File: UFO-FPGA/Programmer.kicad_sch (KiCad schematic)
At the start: 38 parts, among them U2 FT2232HL, U3 ASDMB-12MHz, U5 93LC56CT-I/MS

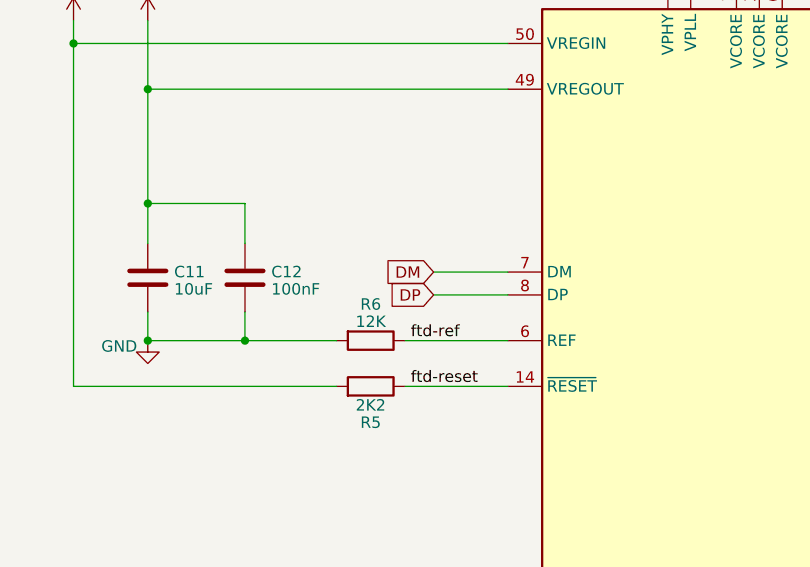
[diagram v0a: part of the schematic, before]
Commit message: pcb prog redesign
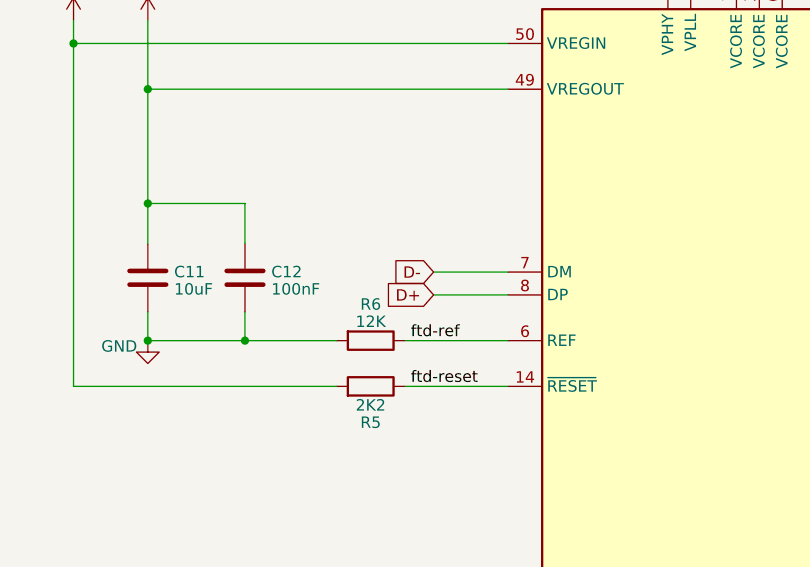
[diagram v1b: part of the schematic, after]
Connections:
- net DM renamed D-
- net DP renamed D+
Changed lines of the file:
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@@
     )
   )
-  (global_label "DP" (shape input) (at 215.265 109.22 180) (fields_autoplaced)
+  (global_label "D+" (shape input) (at 215.265 109.22 180) (fields_autoplaced)
     (effects (font (size 1.27 1.27)) (justify right))
-    (property "Intersheetrefs" "${INTERSHEET_REFS}" (at 209.8192 109.22 0)
+    (property "Intersheetrefs" "${INTERSHEET_REFS}" (at 209.5168 109.22 0)
       (effects (font (size 1.27 1.27)) (justify right) hide)
     )
@@
     )
   )
-  (global_label "DM" (shape input) (at 215.265 106.68 180) (fields_autoplaced)
+  (global_label "D-" (shape input) (at 215.265 106.68 180) (fields_autoplaced)
     (effects (font (size 1.27 1.27)) (justify right))
-    (property "Intersheetrefs" "${INTERSHEET_REFS}" (at 209.6378 106.68 0)
+    (property "Intersheetrefs" "${INTERSHEET_REFS}" (at 209.5168 106.68 0)
       (effects (font (size 1.27 1.27)) (justify right) hide)
     )

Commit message: pcb 0603
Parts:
- C1, C12, C13, C2, C3, C4, C7, C8: footprint Capacitor_SMD:C_0805_2012Metric_Pad1.18x1.45mm_HandSolder -> Capacitor_SMD:C_0603_1608Metric_Pad1.08x0.95mm_HandSolder
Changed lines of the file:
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@@
       (effects (font (size 1.27 1.27)) (justify left))
     )
-    (property "Footprint" "Capacitor_SMD:C_0805_2012Metric_Pad1.18x1.45mm_HandSolder" (at 207.3402 36.83 0)
+    (property "Footprint" "Capacitor_SMD:C_0603_1608Metric_Pad1.08x0.95mm_HandSolder" (at 207.3402 36.83 0)
       (effects (font (size 1.27 1.27)) hide)
     )
@@
       (effects (font (size 1.27 1.27)) (justify right))
     )
-    (property "Footprint" "Capacitor_SMD:C_0805_2012Metric_Pad1.18x1.45mm_HandSolder" (at 249.8598 37.465 0)
+    (property "Footprint" "Capacitor_SMD:C_0603_1608Metric_Pad1.08x0.95mm_HandSolder" (at 249.8598 37.465 0)
       (effects (font (size 1.27 1.27)) hide)
     )
@@
       (effects (font (size 1.27 1.27)) (justify left))
     )
-    (property "Footprint" "Capacitor_SMD:C_0805_2012Metric_Pad1.18x1.45mm_HandSolder" (at 198.4502 36.83 0)
+    (property "Footprint" "Capacitor_SMD:C_0603_1608Metric_Pad1.08x0.95mm_HandSolder" (at 198.4502 36.83 0)
       (effects (font (size 1.27 1.27)) hide)
     )
@@
       (effects (font (size 1.27 1.27)) (justify left))
     )
-    (property "Footprint" "Capacitor_SMD:C_0805_2012Metric_Pad1.18x1.45mm_HandSolder" (at 195.2752 111.125 0)
+    (property "Footprint" "Capacitor_SMD:C_0603_1608Metric_Pad1.08x0.95mm_HandSolder" (at 195.2752 111.125 0)
       (effects (font (size 1.27 1.27)) hide)
     )
@@
       (effects (font (size 1.27 1.27)) (justify left))
     )
-    (property "Footprint" "Capacitor_SMD:C_0805_2012Metric_Pad1.18x1.45mm_HandSolder" (at 86.0552 160.02 0)
+    (property "Footprint" "Capacitor_SMD:C_0603_1608Metric_Pad1.08x0.95mm_HandSolder" (at 86.0552 160.02 0)
       (effects (font (size 1.27 1.27)) hide)
     )
@@
       (effects (font (size 1.27 1.27)) (justify left))
     )
-    (property "Footprint" "Capacitor_SMD:C_0805_2012Metric_Pad1.18x1.45mm_HandSolder" (at 180.0352 175.895 0)
+    (property "Footprint" "Capacitor_SMD:C_0603_1608Metric_Pad1.08x0.95mm_HandSolder" (at 180.0352 175.895 0)
       (effects (font (size 1.27 1.27)) hide)
     )
@@
       (effects (font (size 1.27 1.27)) (justify left))
     )
-    (property "Footprint" "Capacitor_SMD:C_0805_2012Metric_Pad1.18x1.45mm_HandSolder" (at 189.5602 36.83 0)
+    (property "Footprint" "Capacitor_SMD:C_0603_1608Metric_Pad1.08x0.95mm_HandSolder" (at 189.5602 36.83 0)
       (effects (font (size 1.27 1.27)) hide)
     )
@@
       (effects (font (size 1.27 1.27)) (justify left))
     )
-    (property "Footprint" "Capacitor_SMD:C_0805_2012Metric_Pad1.18x1.45mm_HandSolder" (at 232.7402 36.83 0)
-      (effects (font (size 1.27 1.27)) hide)
-    )
+    (property "Footprint" "Capacitor_SMD:C_0603_1608Metric_Pad1.08x0.95mm_HandSolder" (at 232.7402 36.83 0)
+      (effects (font (size 1.27 1.27)) hide)
+    )

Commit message: pcb and footprints
0603
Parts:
- R10, R11, R12, R13, R14, R15, R16, R17, R18, R19, R20, R7, R8, R9: footprint Resistor_SMD:R_0805_2012Metric_Pad1.20x1.40mm_HandSolder -> Resistor_SMD:R_0603_1608Metric_Pad0.98x0.95mm_HandSolder
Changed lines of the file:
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@@
       (effects (font (size 1.27 1.27)))
     )
-    (property "Footprint" "Resistor_SMD:R_0805_2012Metric_Pad1.20x1.40mm_HandSolder" (at 307.34 144.018 90)
+    (property "Footprint" "Resistor_SMD:R_0603_1608Metric_Pad0.98x0.95mm_HandSolder" (at 307.34 144.018 90)
       (effects (font (size 1.27 1.27)) hide)
     )
@@
       (effects (font (size 1.27 1.27)))
     )
-    (property "Footprint" "Resistor_SMD:R_0805_2012Metric_Pad1.20x1.40mm_HandSolder" (at 307.34 100.838 90)
+    (property "Footprint" "Resistor_SMD:R_0603_1608Metric_Pad0.98x0.95mm_HandSolder" (at 307.34 100.838 90)
       (effects (font (size 1.27 1.27)) hide)
     )
@@
       (effects (font (size 1.27 1.27)))
     )
-    (property "Footprint" "Resistor_SMD:R_0805_2012Metric_Pad1.20x1.40mm_HandSolder" (at 307.34 131.318 90)
+    (property "Footprint" "Resistor_SMD:R_0603_1608Metric_Pad0.98x0.95mm_HandSolder" (at 307.34 131.318 90)
       (effects (font (size 1.27 1.27)) hide)
     )
@@
       (effects (font (size 1.27 1.27)))
     )
-    (property "Footprint" "Resistor_SMD:R_0805_2012Metric_Pad1.20x1.40mm_HandSolder" (at 307.34 93.218 90)
+    (property "Footprint" "Resistor_SMD:R_0603_1608Metric_Pad0.98x0.95mm_HandSolder" (at 307.34 93.218 90)
       (effects (font (size 1.27 1.27)) hide)
     )
@@
       (effects (font (size 1.27 1.27)))
     )
-    (property "Footprint" "Resistor_SMD:R_0805_2012Metric_Pad1.20x1.40mm_HandSolder" (at 307.34 128.778 90)
+    (property "Footprint" "Resistor_SMD:R_0603_1608Metric_Pad0.98x0.95mm_HandSolder" (at 307.34 128.778 90)
       (effects (font (size 1.27 1.27)) hide)
     )
@@
       (effects (font (size 1.27 1.27)))
     )
-    (property "Footprint" "Resistor_SMD:R_0805_2012Metric_Pad1.20x1.40mm_HandSolder" (at 307.34 85.598 90)
+    (property "Footprint" "Resistor_SMD:R_0603_1608Metric_Pad0.98x0.95mm_HandSolder" (at 307.34 85.598 90)
       (effects (font (size 1.27 1.27)) hide)
     )
@@
       (effects (font (size 1.27 1.27)))
     )
-    (property "Footprint" "Resistor_SMD:R_0805_2012Metric_Pad1.20x1.40mm_HandSolder" (at 307.34 88.138 90)
+    (property "Footprint" "Resistor_SMD:R_0603_1608Metric_Pad0.98x0.95mm_HandSolder" (at 307.34 88.138 90)
       (effects (font (size 1.27 1.27)) hide)
     )
@@
       (effects (font (size 1.27 1.27)))
     )
-    (property "Footprint" "Resistor_SMD:R_0805_2012Metric_Pad1.20x1.40mm_HandSolder" (at 307.34 83.058 90)
+    (property "Footprint" "Resistor_SMD:R_0603_1608Metric_Pad0.98x0.95mm_HandSolder" (at 307.34 83.058 90)
       (effects (font (size 1.27 1.27)) hide)
     )
@@
       (effects (font (size 1.27 1.27)))
     )
-    (property "Footprint" "Resistor_SMD:R_0805_2012Metric_Pad1.20x1.40mm_HandSolder" (at 307.34 138.938 90)
+    (property "Footprint" "Resistor_SMD:R_0603_1608Metric_Pad0.98x0.95mm_HandSolder" (at 307.34 138.938 90)
       (effects (font (size 1.27 1.27)) hide)
     )
@@
       (effects (font (size 1.27 1.27)))
     )
-    (property "Footprint" "Resistor_SMD:R_0805_2012Metric_Pad1.20x1.40mm_HandSolder" (at 184.785 193.548 90)
+    (property "Footprint" "Resistor_SMD:R_0603_1608Metric_Pad0.98x0.95mm_HandSolder" (at 184.785 193.548 90)
       (effects (font (size 1.27 1.27)) hide)
     )
@@
       (effects (font (size 1.27 1.27)))
     )
-    (property "Footprint" "Resistor_SMD:R_0805_2012Metric_Pad1.20x1.40mm_HandSolder" (at 307.34 141.478 90)
+    (property "Footprint" "Resistor_SMD:R_0603_1608Metric_Pad0.98x0.95mm_HandSolder" (at 307.34 141.478 90)
       (effects (font (size 1.27 1.27)) hide)
     )
@@
       (effects (font (size 1.27 1.27)))
     )
-    (property "Footprint" "Resistor_SMD:R_0805_2012Metric_Pad1.20x1.40mm_HandSolder" (at 307.34 98.298 90)
+    (property "Footprint" "Resistor_SMD:R_0603_1608Metric_Pad0.98x0.95mm_HandSolder" (at 307.34 98.298 90)
       (effects (font (size 1.27 1.27)) hide)
     )
@@
       (effects (font (size 1.27 1.27)))
     )
-    (property "Footprint" "Resistor_SMD:R_0805_2012Metric_Pad1.20x1.40mm_HandSolder" (at 307.34 133.858 90)
+    (property "Footprint" "Resistor_SMD:R_0603_1608Metric_Pad0.98x0.95mm_HandSolder" (at 307.34 133.858 90)
       (effects (font (size 1.27 1.27)) hide)
     )
@@
       (effects (font (size 1.27 1.27)))
     )
-    (property "Footprint" "Resistor_SMD:R_0805_2012Metric_Pad1.20x1.40mm_HandSolder" (at 307.34 136.398 90)
-      (effects (font (size 1.27 1.27)) hide)
-    )
+    (property "Footprint" "Resistor_SMD:R_0603_1608Metric_Pad0.98x0.95mm_HandSolder" (at 307.34 136.398 90)
+      (effects (font (size 1.27 1.27)) hide)
+    )

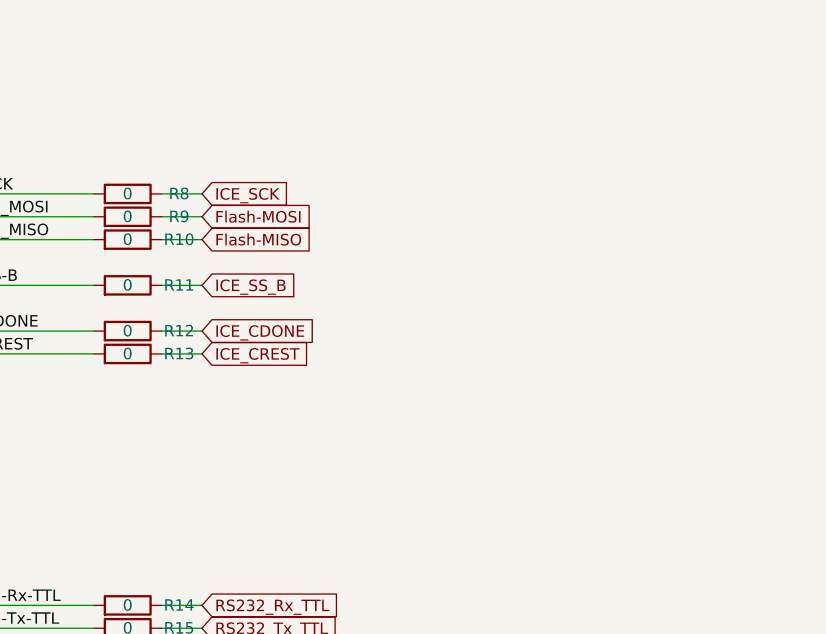
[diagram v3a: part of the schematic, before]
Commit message: pcb
added John zendong
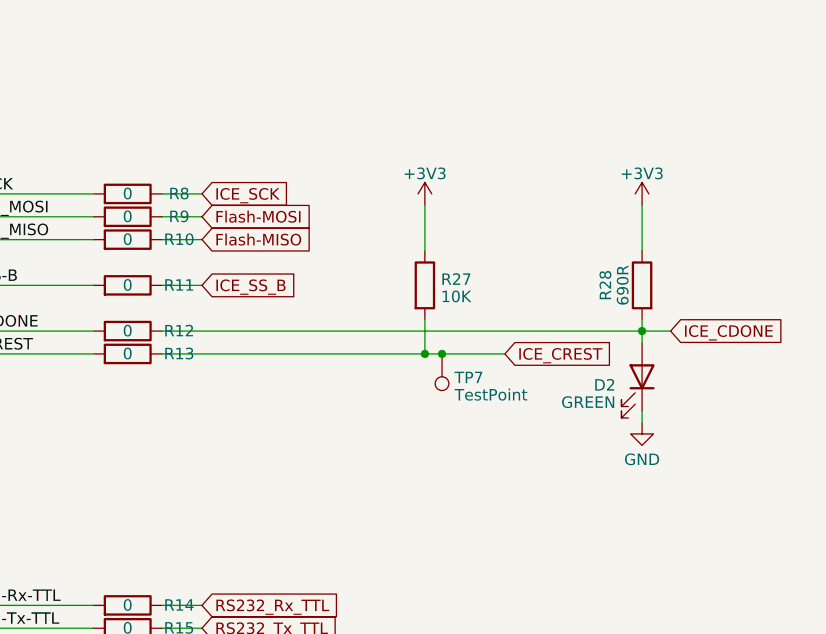
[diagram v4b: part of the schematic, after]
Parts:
- added D2: GREEN, LED_SMD:LED_0805_2012Metric_Pad1.15x1.40mm_HandSolder, symbol Device:LED
- added R27: 10K, Resistor_SMD:R_0603_1608Metric_Pad0.98x0.95mm_HandSolder, symbol Device:R
- added R28: 690R, Resistor_SMD:R_0805_2012Metric_Pad1.20x1.40mm_HandSolder, symbol Device:R
- added TP7: TestPoint, TestPoint:TestPoint_Pad_1.5x1.5mm, symbol Connector:TestPoint
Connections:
- net +3V3: now also R27.1, R28.1
- net GND: now also D2.1 (K)
- net ICE_CDONE: now also D2.2 (A), R28.2
- net ICE_CREST: now also R27.2, TP7.1
